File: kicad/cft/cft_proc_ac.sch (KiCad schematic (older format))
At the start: 24 parts, among them U504 74HCT541, U506 74HCT541, U509 74HCT541, U601 74HCT541, U602 74HC193, U603 74HCT541, U604 74HC193, U605 74HCT541, U606 74HC193, U607 74HC688, U608 74HCT541, U609 74HC193, U610 74HC688, U612 74AHC1G08

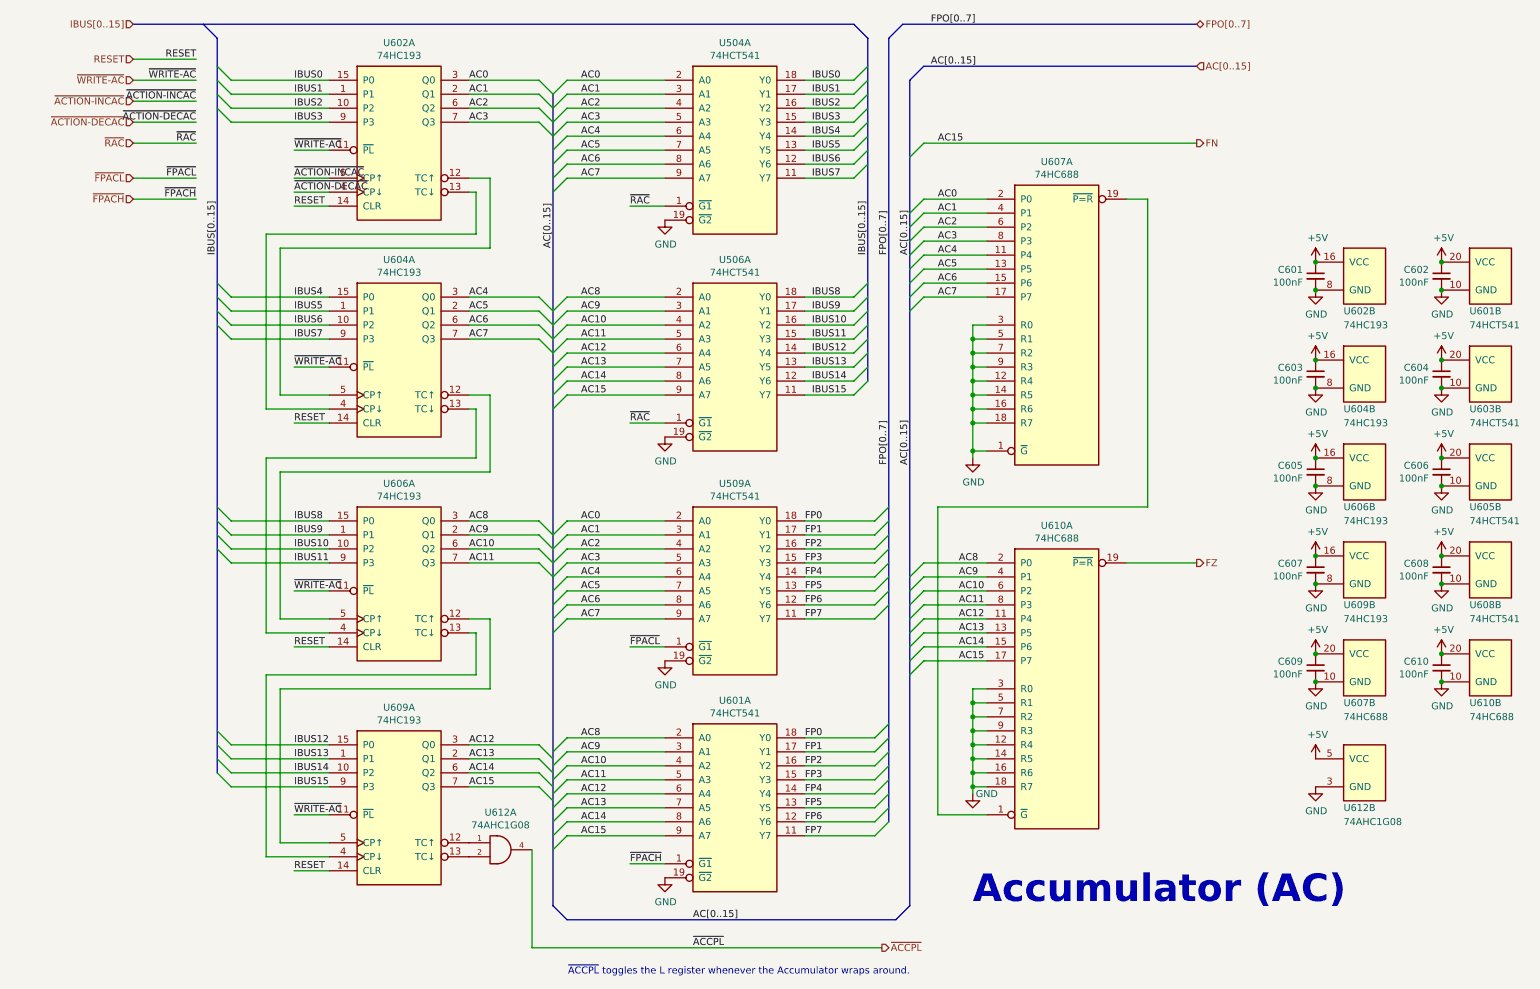
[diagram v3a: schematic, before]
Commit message: Moved things around a bit
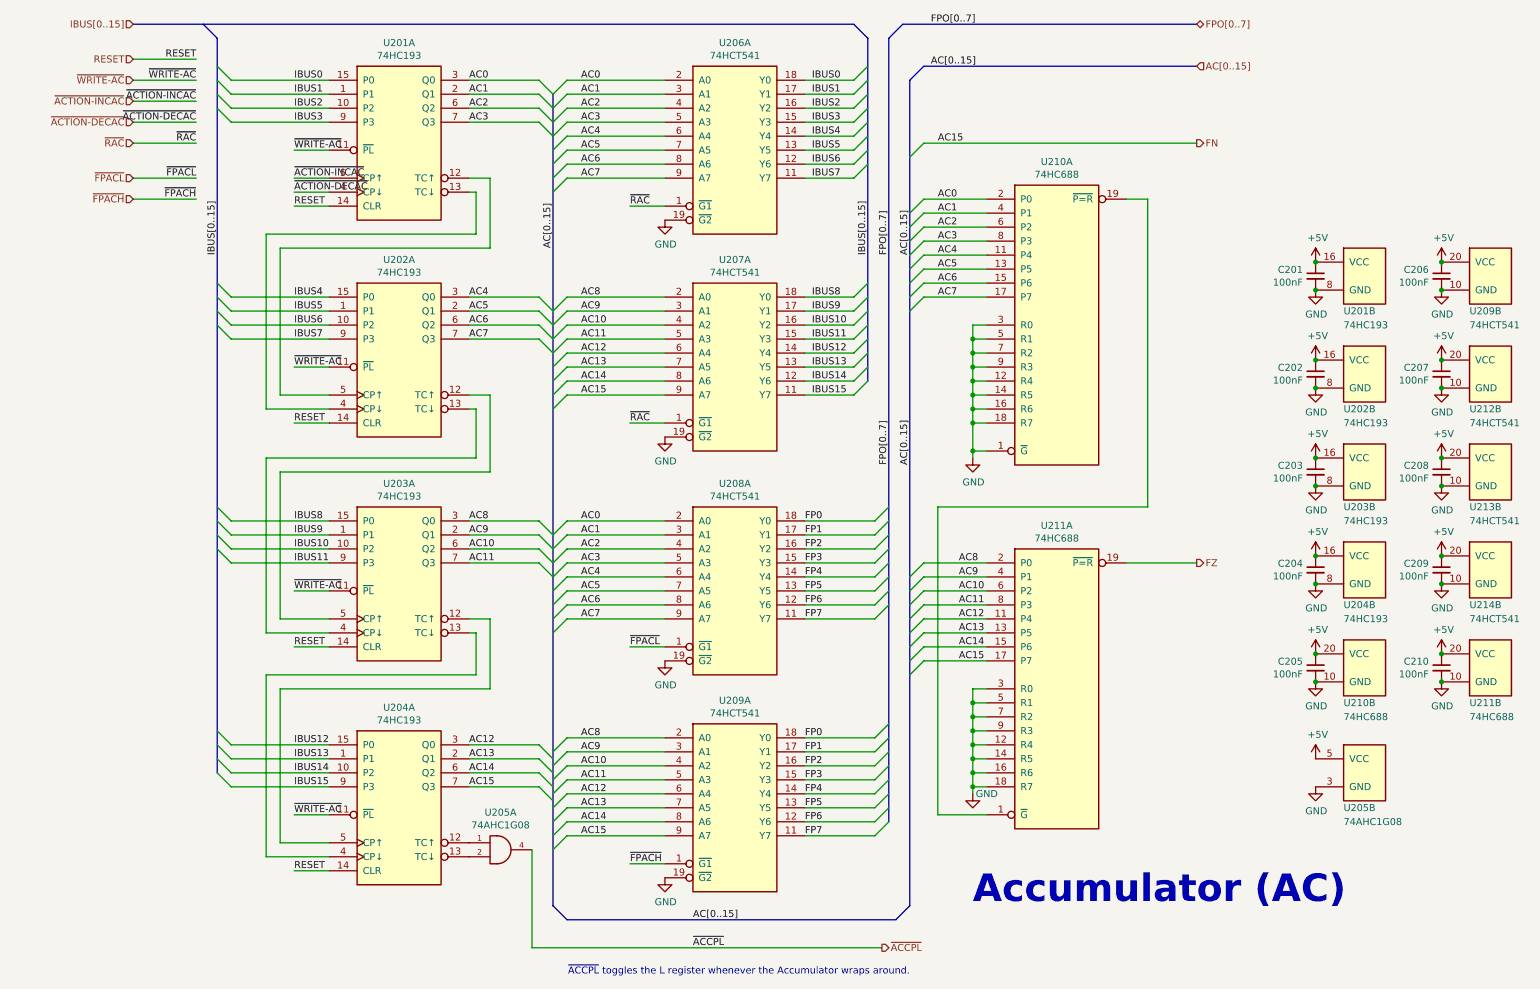
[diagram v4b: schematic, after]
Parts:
- renumbered C601 to C201, C603 to C202, C605 to C203, C607 to C204, C609 to C205, C602 to C206, C604 to C207, C606 to C208, C608 to C209, C610 to C210, U602 to U201, U604 to U202, U606 to U203, U609 to U204, U612 to U205, U504 to U206, U506 to U207, U509 to U208, U601 to U209, U607 to U210, U610 to U211, U603 to U212, U605 to U213, U608 to U214

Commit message: Removed widebus buffer from microcode store µAddr High
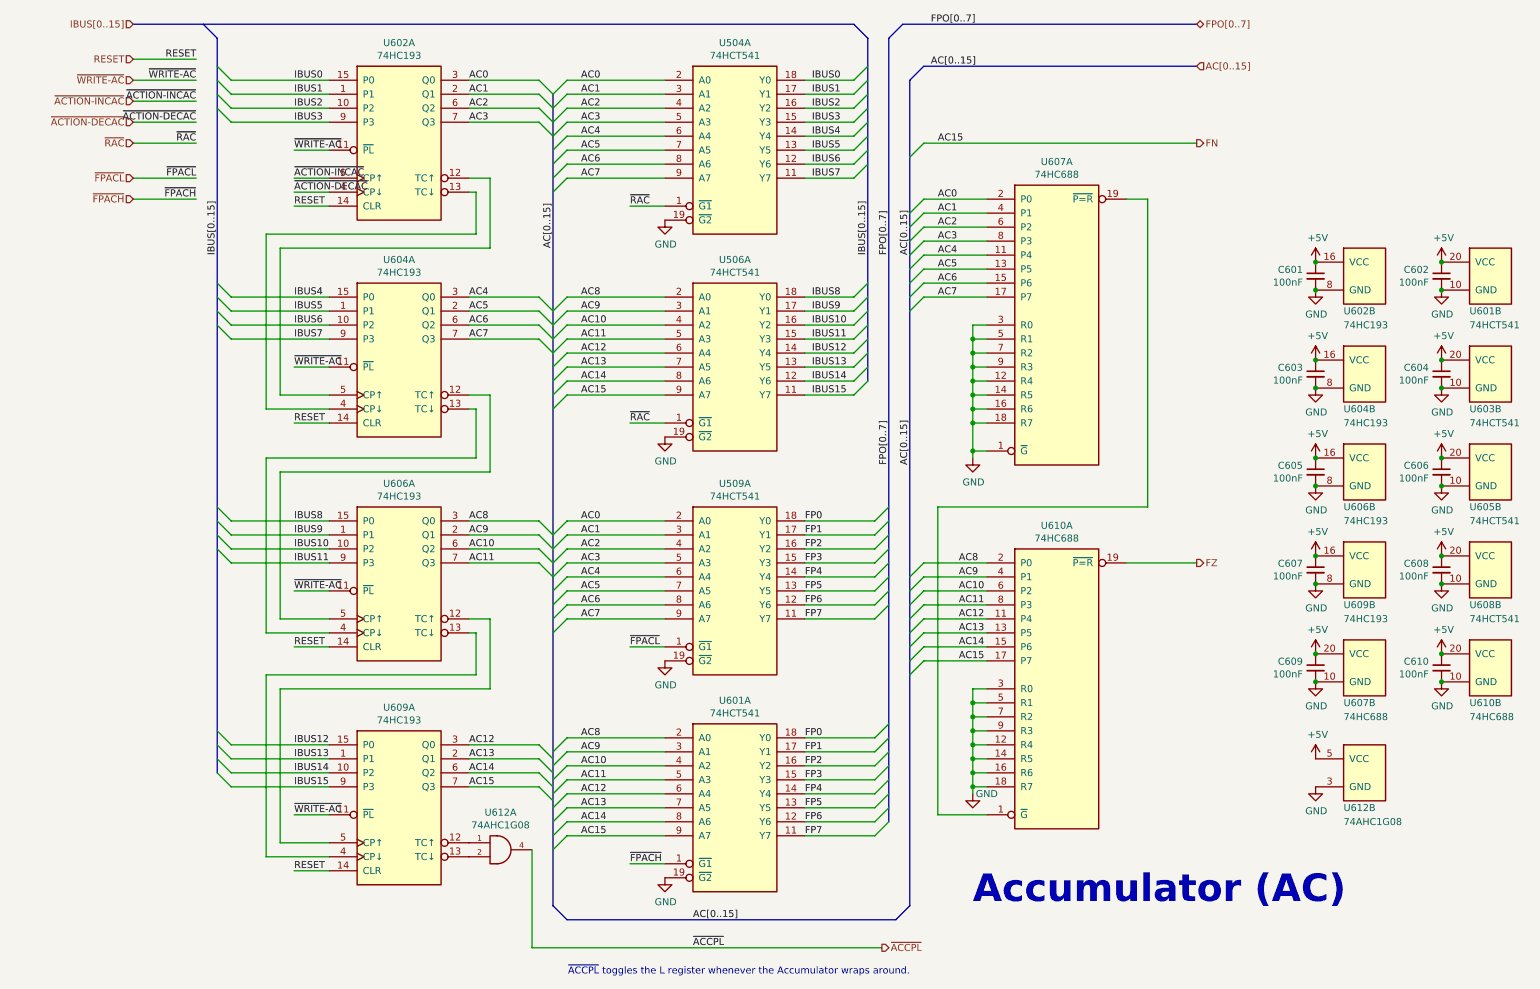
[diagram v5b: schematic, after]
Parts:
- renumbered C201 to C601, C206 to C602, C202 to C603, C207 to C604, C203 to C605, C208 to C606, C204 to C607, C209 to C608, C205 to C609, C210 to C610, U206 to U504, U207 to U506, U208 to U509, U209 to U601, U201 to U602, U212 to U603, U202 to U604, U213 to U605, U203 to U606, U210 to U607, U214 to U608, U204 to U609, U211 to U610, U205 to U612
